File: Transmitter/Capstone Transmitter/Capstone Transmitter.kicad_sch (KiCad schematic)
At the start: 5 parts, among them U1 ESP32-C3-DevKitM-1, U2 TPS63020DSJR

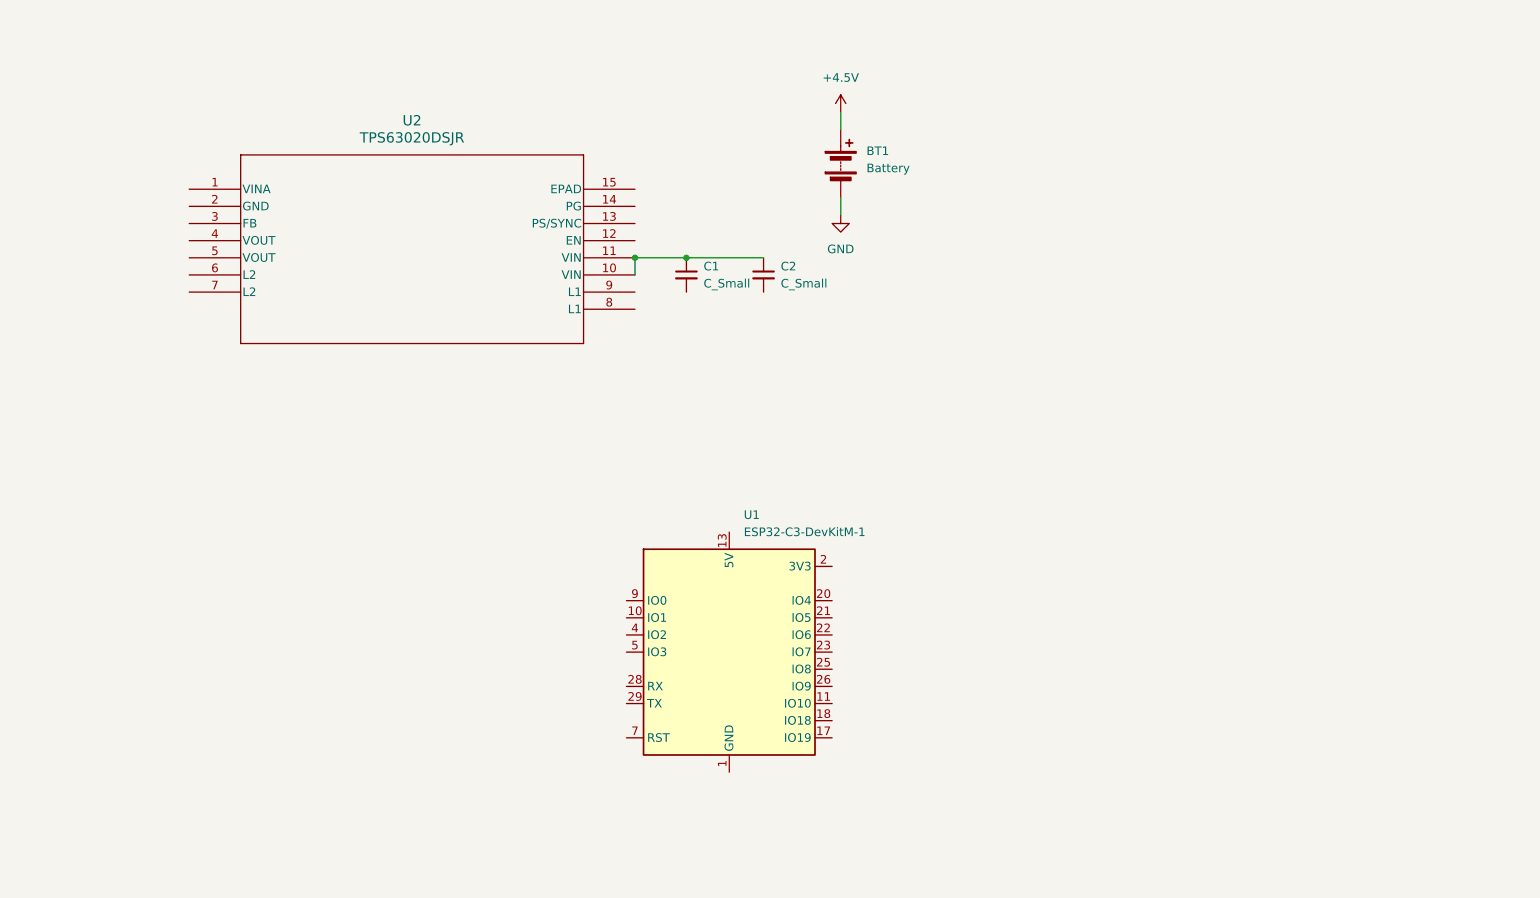
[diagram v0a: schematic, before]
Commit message: WIP remote
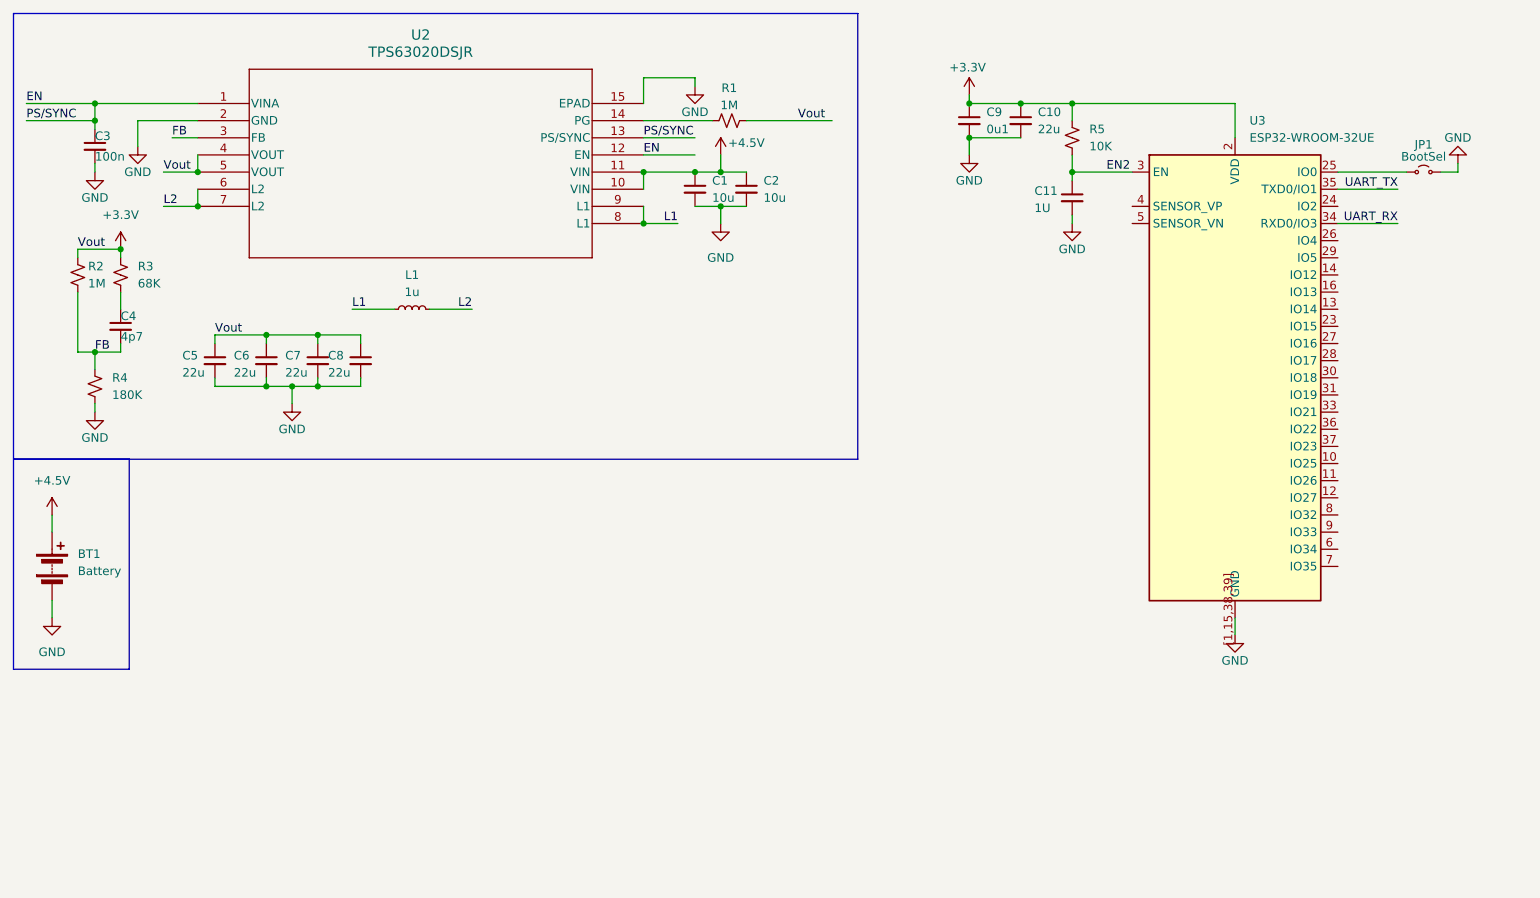
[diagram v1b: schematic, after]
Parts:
- removed U1: ESP32-C3-DevKitM-1, RF_Module:ESP32-C3-DevKitM-1, symbol RF_Module:ESP32-C3-DevKitM-1
- added C10, C5, C6, C7, C8: 22u, symbol Device:C_Small
- added C11: 1U, symbol Device:C_Small
- added C3: 100n, symbol Device:C_Small
- added C4: 4p7, symbol Device:C_Small
- added C9: 0u1, symbol Device:C_Small
- added JP1: BootSel, symbol Jumper:Jumper_2_Small_Open
- added L1: 1u, symbol Device:L_Small
- added R1, R2: 1M, symbol Device:R_Small_US
- added R3: 68K, symbol Device:R_Small_US
- added R4: 180K, symbol Device:R_Small_US
- added R5: 10K, symbol Device:R_Small_US
- added U3: ESP32-WROOM-32UE, RF_Module:ESP32-WROOM-32UE, symbol RF_Module:ESP32-WROOM-32UE
- C1, C2: value C_Small -> 10u
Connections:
- net +4.5V: now also C1.1, C2.1, U2.10 (VIN), U2.11 (VIN)
- net GND: now also C1.2, C2.2, U2.15 (EPAD), U2.2 (GND), C10.2, C11.2, C3.2, C5.2, C6.2, C7.2, C8.2, C9.2, JP1.2 (B), R4.2, U3.[1,15,38,39] (GND)
- net EN: now reaches U2.1 (VINA)
- net EN: now also U2.12 (EN), C3.1
- net PS/SYNC: now reaches U2.13 (PS/SYNC)
- net at U2.14 (PG): now also R1.1
- net FB: now reaches U2.3 (FB)
- net FB: now also C4.2, R2.2, R4.1
- net +3.3V: now reaches U2.4 (VOUT)
- net +3.3V: now also U2.5 (VOUT), C10.1, C5.1, C6.1, C7.1, C8.1, C9.1, R1.2, R2.1, R3.1, R5.1, U3.2 (VDD)
- net L2: now reaches U2.6 (L2)
- net L2: now also U2.7 (L2), L1.2
- net L1: now reaches U2.8 (L1)
- net L1: now also U2.9 (L1), L1.1
- new net: JP1.1 (A), U3.25 (IO0)
- new net: C4.1, R3.2
- new net EN2: C11.1, R5.2, U3.3 (EN)
- new net UART_RX: U3.34 (RXD0/IO3)
- new net UART_TX: U3.35 (TXD0/IO1)
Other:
- moved on the sheet: BT1, C1, C2, U2

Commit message: Finished remote schematic, getting some sleep now
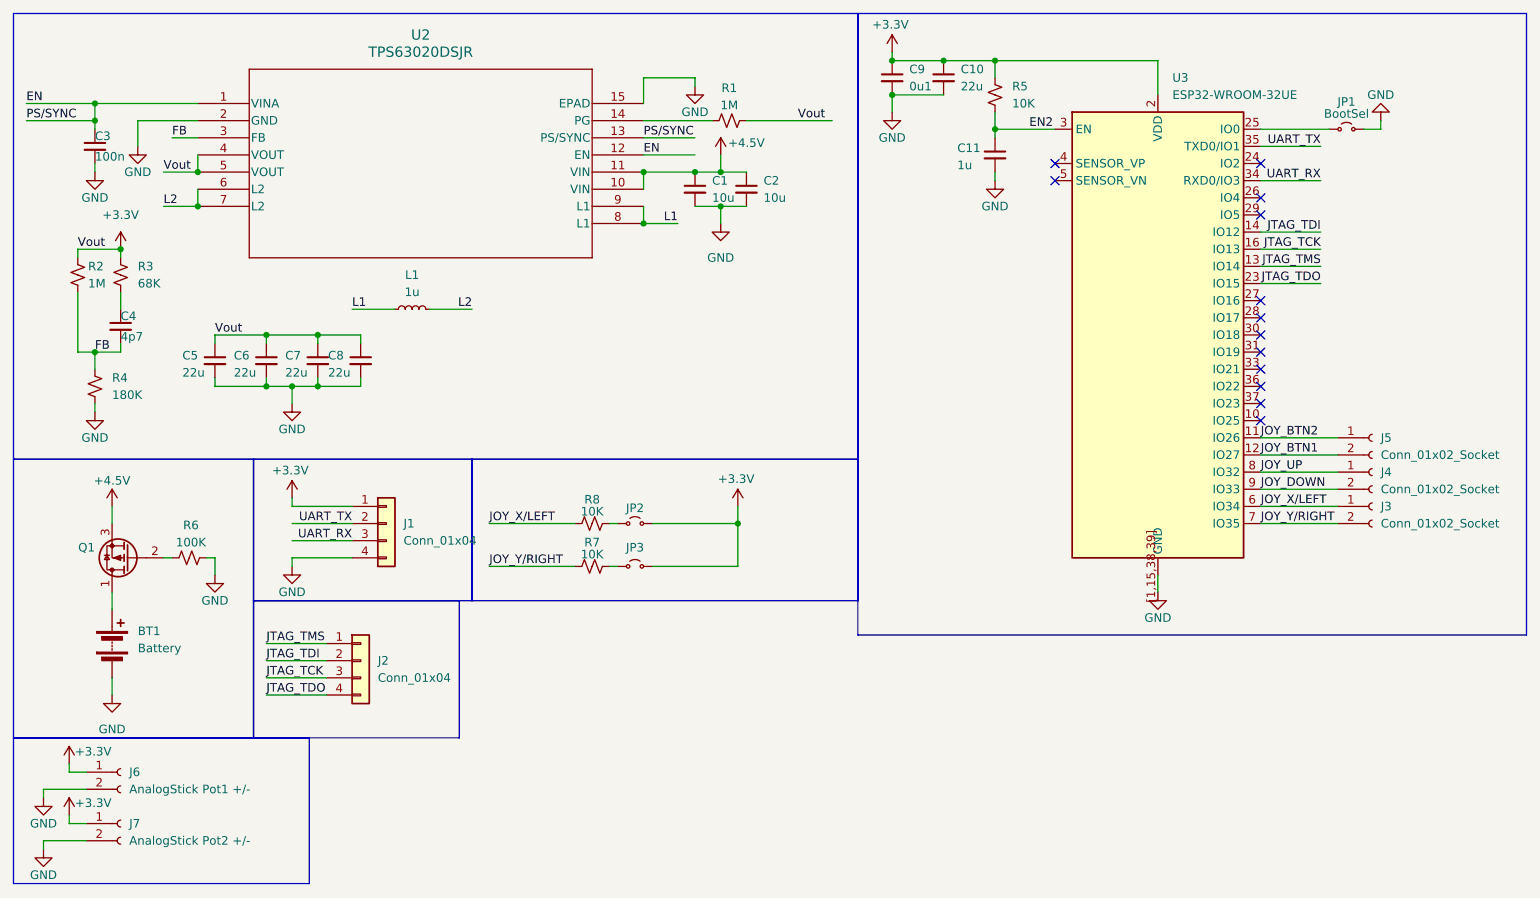
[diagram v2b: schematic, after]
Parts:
- added J1, J2: Conn_01x04, symbol Connector_Generic:Conn_01x04
- added J3, J4, J5: Conn_01x02_Socket, symbol Connector:Conn_01x02_Socket
- added J6: AnalogStick Pot1 +/-, symbol Connector:Conn_01x02_Socket
- added J7: AnalogStick Pot2 +/-, symbol Connector:Conn_01x02_Socket
- added JP2: Pull up Jumper 1, symbol Jumper:Jumper_2_Small_Open
- added JP3: Pull up Jumper 2, symbol Jumper:Jumper_2_Small_Open
- added Q1: RevPolProt, symbol Transistor_FET:Q_PMOS_DGS
- added R6: 100K, symbol Device:R_Small_US
- added R7, R8: 10K, symbol Device:R_Small_US
- C11: value 1U -> 1u
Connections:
- net +3.3V: now also J1.1 (Pin_1), J6.1 (Pin_1), J7.1 (Pin_1), JP2.2 (B), JP3.2 (B)
- net +4.5V: now also Q1.3 (S); no longer BT1.1 (+)
- net GND: now also J1.4 (Pin_4), J6.2 (Pin_2), J7.2 (Pin_2), R6.2
- net UART_RX: now also J1.3 (Pin_3)
- net UART_TX: now also J1.2 (Pin_2)
- net JOY_BTN2: now reaches U3.11 (IO26)
- net JOY_BTN2: now also J5.1 (Pin_1)
- net JOY_BTN1: now reaches U3.12 (IO27)
- net JOY_BTN1: now also J5.2 (Pin_2)
- net JTAG_TMS: now reaches U3.13 (IO14)
- net JTAG_TMS: now also J2.1 (Pin_1)
- net JTAG_TDI: now reaches U3.14 (IO12)
- net JTAG_TDI: now also J2.2 (Pin_2)
- net JTAG_TCK: now reaches U3.16 (IO13)
- net JTAG_TCK: now also J2.3 (Pin_3)
- net JTAG_TDO: now reaches U3.23 (IO15)
- net JTAG_TDO: now also J2.4 (Pin_4)
- net JOY_X/LEFT: now reaches U3.6 (IO34)
- net JOY_X/LEFT: now also J3.1 (Pin_1), R8.1
- net JOY_Y/RIGHT: now reaches U3.7 (IO35)
- net JOY_Y/RIGHT: now also J3.2 (Pin_2), R7.1
- net JOY_UP: now reaches U3.8 (IO32)
- net JOY_UP: now also J4.1 (Pin_1)
- net JOY_DOWN: now reaches U3.9 (IO33)
- net JOY_DOWN: now also J4.2 (Pin_2)
- new net: JP2.1 (A), R8.2
- new net: BT1.1 (+), Q1.1 (D)
- new net: Q1.2 (G), R6.1
- new net: JP3.1 (A), R7.2
- no-connect marks 0 -> 13
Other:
- moved on the sheet: BT1, C10, C11, C9, JP1, R5, U3
